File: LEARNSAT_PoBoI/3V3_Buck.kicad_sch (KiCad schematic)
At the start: 22 parts, among them U5 LT1616ES6#TRMPBF, U7 LT1616ES6#TRMPBF

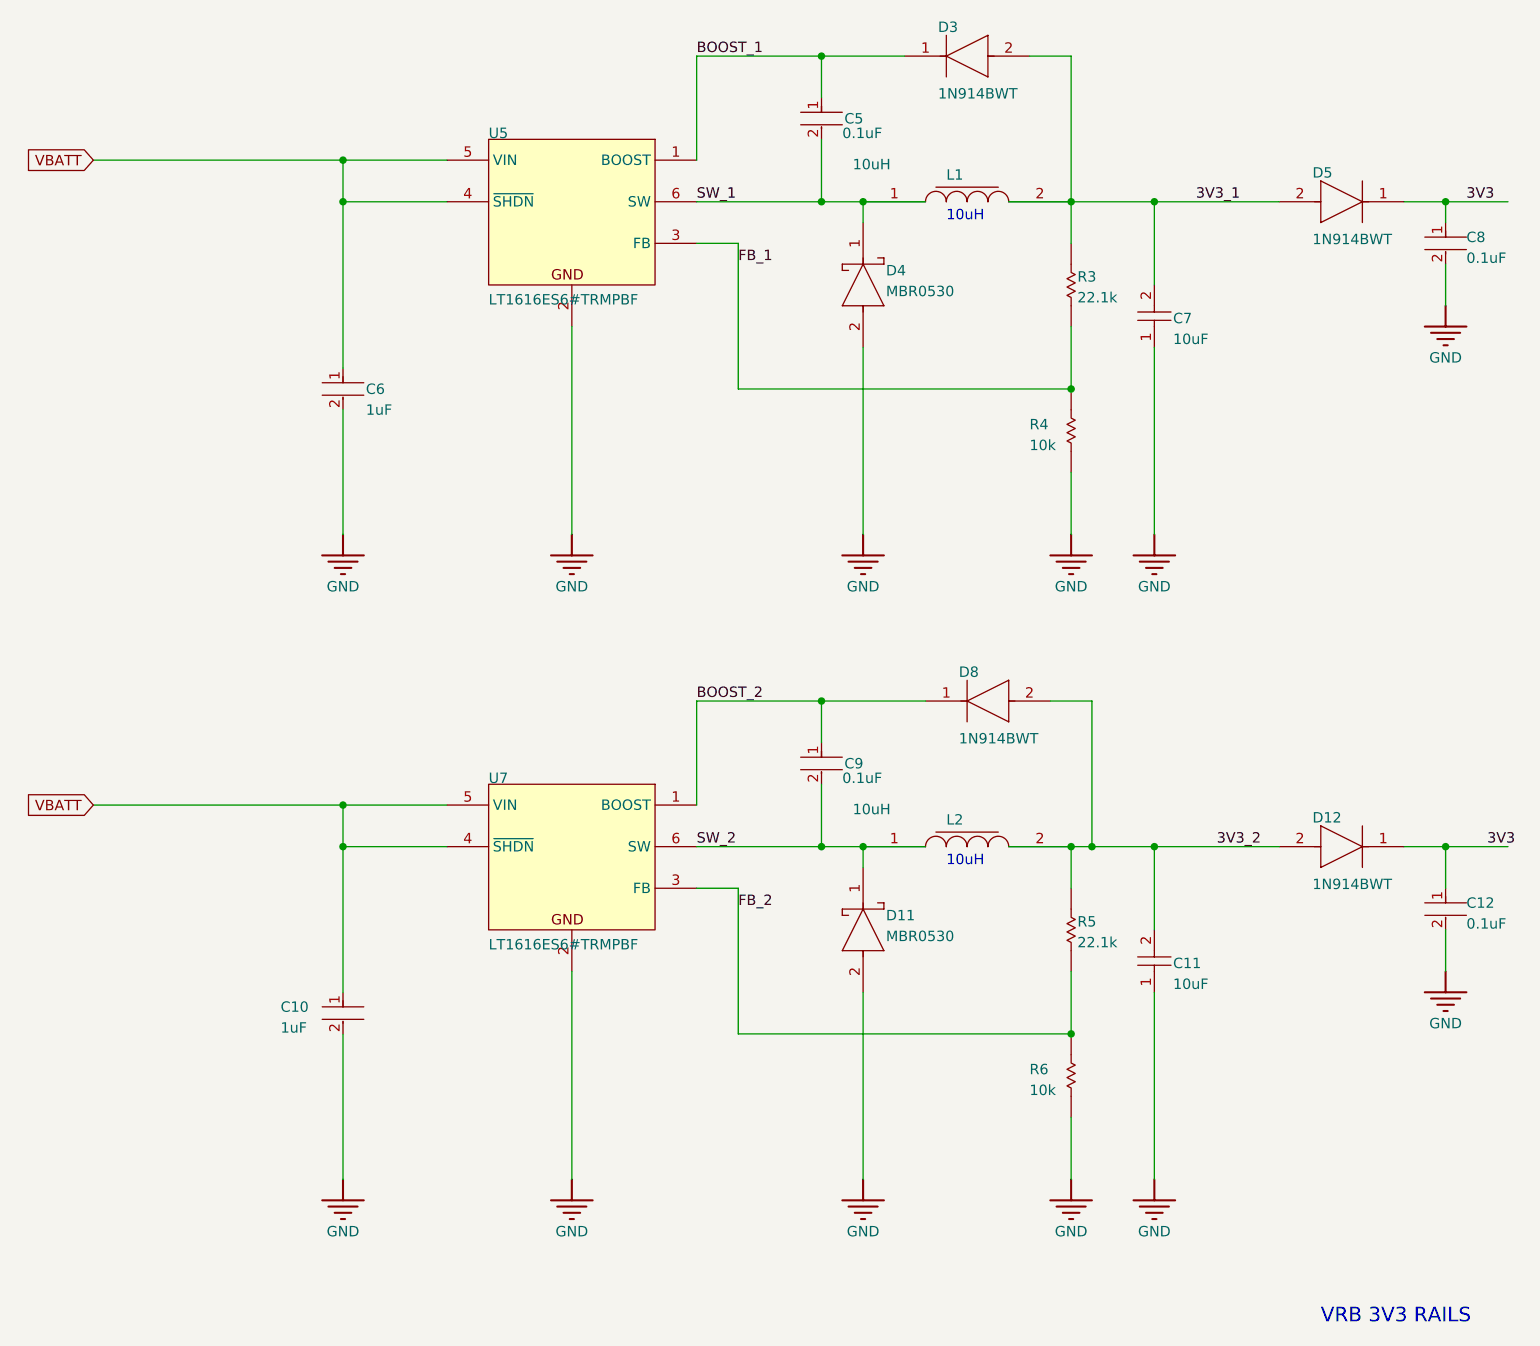
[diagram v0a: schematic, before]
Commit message: Added footprints
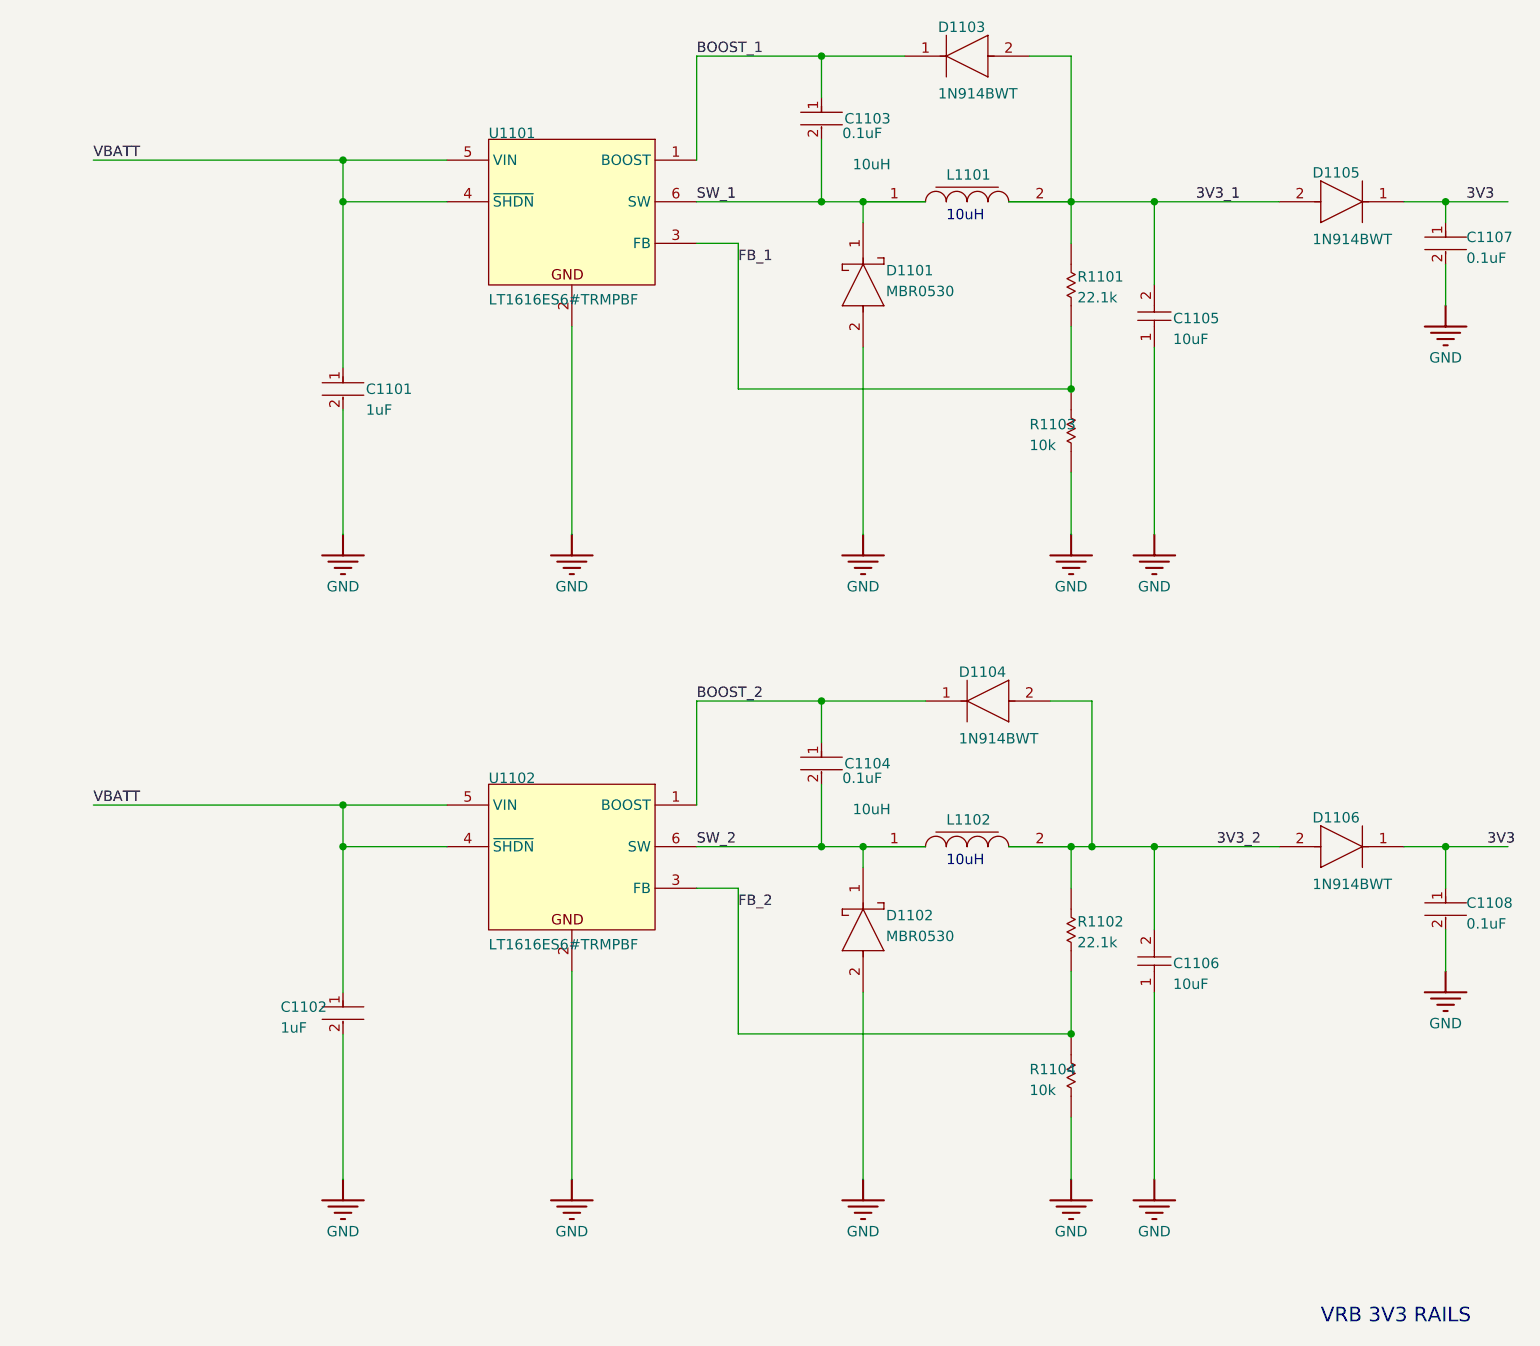
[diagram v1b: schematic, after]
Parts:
- C1101: renamed from C6; footprint FP-CL10-IPC_B -> Capacitor_SMD:C_0603_1608Metric
- C1102: renamed from C10; footprint FP-CL10-IPC_B -> Capacitor_SMD:C_0603_1608Metric
- C1103: renamed from C5; footprint FP-C0603-CJ-MFG -> Capacitor_SMD:C_0603_1608Metric
- C1104: renamed from C9; footprint FP-C0603-CJ-MFG -> Capacitor_SMD:C_0603_1608Metric
- C1105: renamed from C7; footprint CAPC0603(1608)100_L -> Capacitor_SMD:C_0603_1608Metric
- C1106: renamed from C11; footprint CAPC0603(1608)100_L -> Capacitor_SMD:C_0603_1608Metric
- C1107: renamed from C8; footprint FP-C0603-CJ-MFG -> Capacitor_SMD:C_0603_1608Metric
- C1108: renamed from C12; footprint FP-C0603-CJ-MFG -> Capacitor_SMD:C_0603_1608Metric
- D1101: renamed from D4; footprint FP-425-04-MFG -> Diode_SMD:D_SOD-123
- D1102: renamed from D11; footprint FP-425-04-MFG -> Diode_SMD:D_SOD-123
- D1103: renamed from D3; footprint FP-502-01-MFG -> Diode_SMD:D_SOD-123
- D1104: renamed from D8; footprint FP-502-01-MFG -> Diode_SMD:D_SOD-123
- D1105: renamed from D5; footprint FP-502-01-MFG -> Diode_SMD:D_SOD-123
- D1106: renamed from D12; footprint FP-502-01-MFG -> Diode_SMD:D_SOD-123
- L1101: renamed from L1; footprint INDM3532X15N -> L110X:L110X
- L1102: renamed from L2; footprint INDM3532X15N -> L110X:L110X
- R1101: renamed from R3; footprint RESC1609X50X30LL10T20 -> Resistor_SMD:R_0603_1608Metric
- R1102: renamed from R5; footprint RESC1609X50X30LL10T20 -> Resistor_SMD:R_0603_1608Metric
- R1103: renamed from R4; footprint RESC1609X50X30NL8T20 -> Resistor_SMD:R_0603_1608Metric
- R1104: renamed from R6; footprint RESC1609X50X30NL8T20 -> Resistor_SMD:R_0603_1608Metric
- U1101: renamed from U5; footprint LT-S6-6-SOT-23_M -> LT1616ES6TRMPBF:SOT-6_S
- U1102: renamed from U7; footprint LT-S6-6-SOT-23_M -> LT1616ES6TRMPBF:SOT-6_S

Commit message: Add files via upload
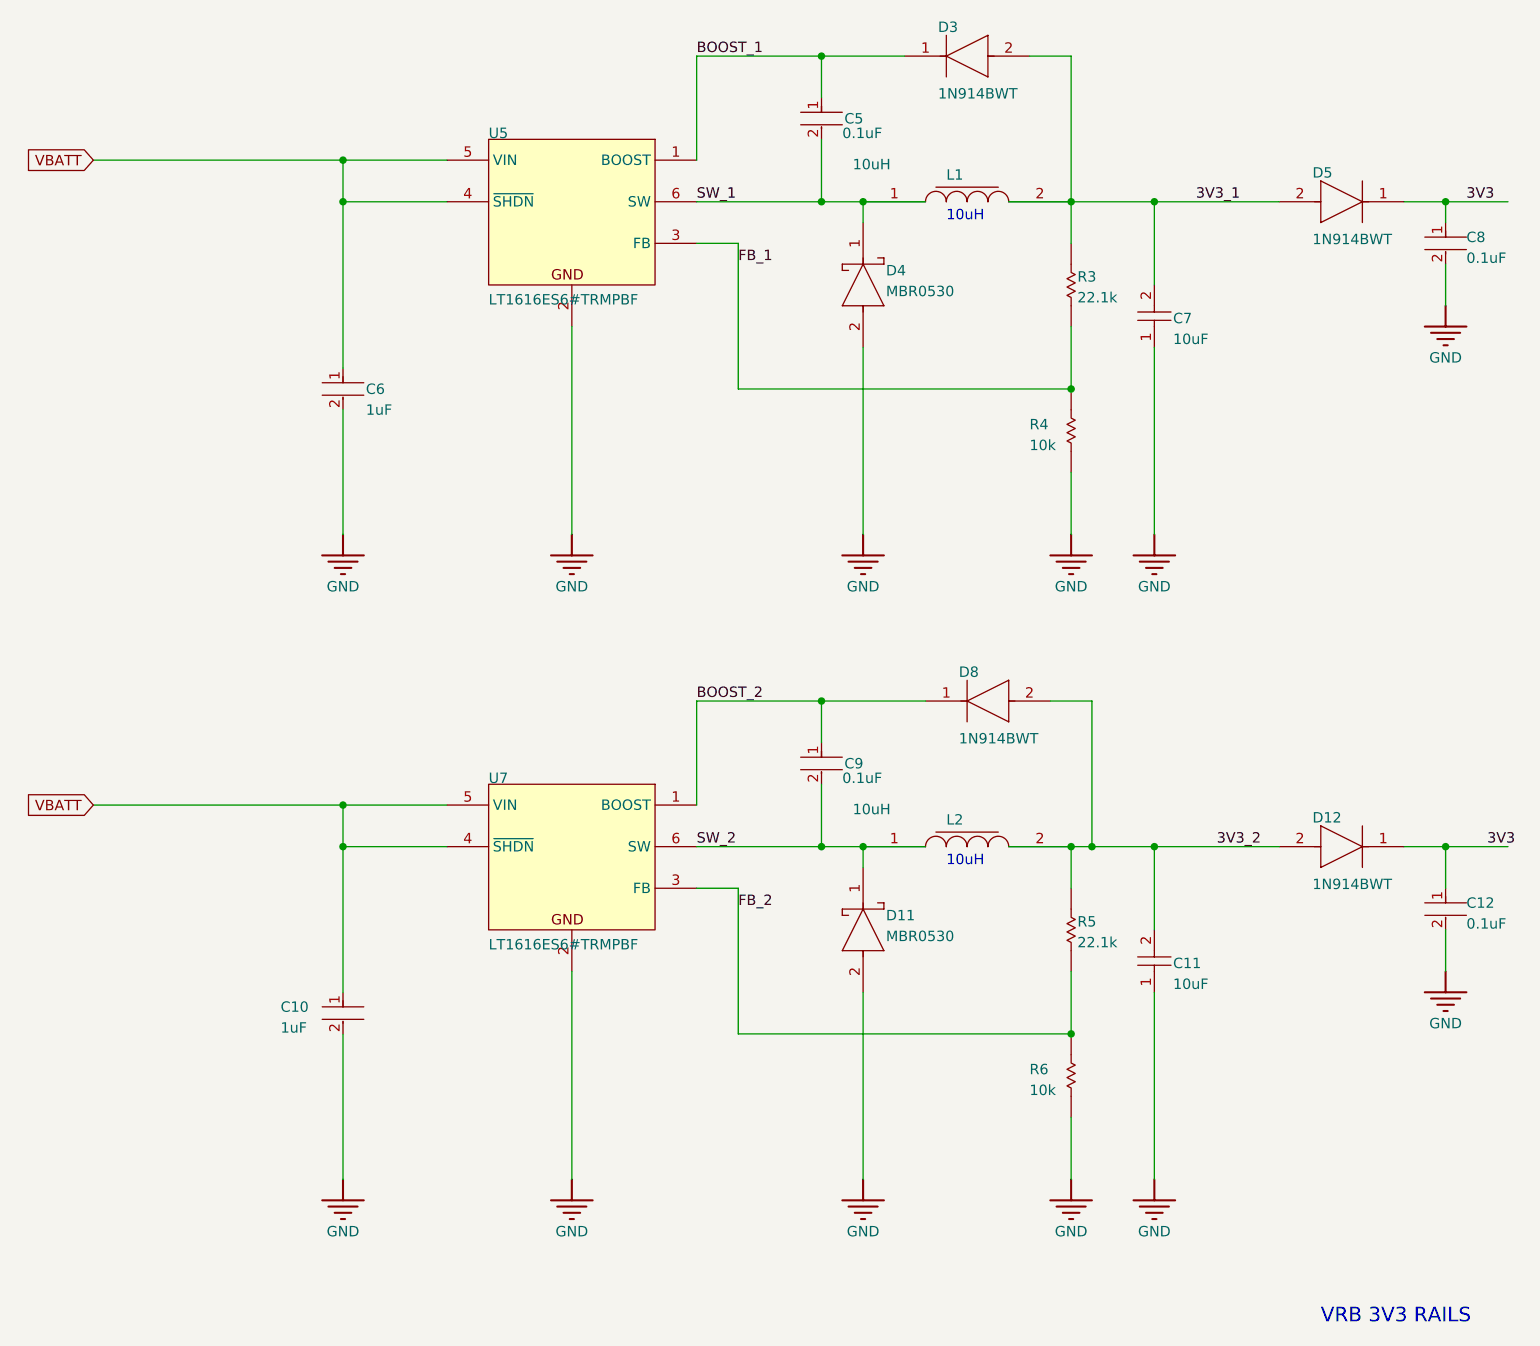
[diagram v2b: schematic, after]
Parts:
- C10: renamed from C1102; footprint Capacitor_SMD:C_0603_1608Metric -> FP-CL10-IPC_B
- C11: renamed from C1106; footprint Capacitor_SMD:C_0603_1608Metric -> CAPC0603(1608)100_L
- C12: renamed from C1108; footprint Capacitor_SMD:C_0603_1608Metric -> FP-C0603-CJ-MFG
- C5: renamed from C1103; footprint Capacitor_SMD:C_0603_1608Metric -> FP-C0603-CJ-MFG
- C6: renamed from C1101; footprint Capacitor_SMD:C_0603_1608Metric -> FP-CL10-IPC_B
- C7: renamed from C1105; footprint Capacitor_SMD:C_0603_1608Metric -> CAPC0603(1608)100_L
- C8: renamed from C1107; footprint Capacitor_SMD:C_0603_1608Metric -> FP-C0603-CJ-MFG
- C9: renamed from C1104; footprint Capacitor_SMD:C_0603_1608Metric -> FP-C0603-CJ-MFG
- D11: renamed from D1102; footprint Diode_SMD:D_SOD-123 -> FP-425-04-MFG
- D12: renamed from D1106; footprint Diode_SMD:D_SOD-123 -> FP-502-01-MFG
- D3: renamed from D1103; footprint Diode_SMD:D_SOD-123 -> FP-502-01-MFG
- D4: renamed from D1101; footprint Diode_SMD:D_SOD-123 -> FP-425-04-MFG
- D5: renamed from D1105; footprint Diode_SMD:D_SOD-123 -> FP-502-01-MFG
- D8: renamed from D1104; footprint Diode_SMD:D_SOD-123 -> FP-502-01-MFG
- L1: renamed from L1101; footprint L110X:L110X -> INDM3532X15N
- L2: renamed from L1102; footprint L110X:L110X -> INDM3532X15N
- R3: renamed from R1101; footprint Resistor_SMD:R_0603_1608Metric -> RESC1609X50X30LL10T20
- R4: renamed from R1103; footprint Resistor_SMD:R_0603_1608Metric -> RESC1609X50X30NL8T20
- R5: renamed from R1102; footprint Resistor_SMD:R_0603_1608Metric -> RESC1609X50X30LL10T20
- R6: renamed from R1104; footprint Resistor_SMD:R_0603_1608Metric -> RESC1609X50X30NL8T20
- U5: renamed from U1101; footprint LT1616ES6TRMPBF:SOT-6_S -> LT-S6-6-SOT-23_M
- U7: renamed from U1102; footprint LT1616ES6TRMPBF:SOT-6_S -> LT-S6-6-SOT-23_M
